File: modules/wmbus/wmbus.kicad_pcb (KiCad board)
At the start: 2 copper layers, 25.4 x 28.6 mm, 15 parts, among them J1 Conn_01x08, J2 Conn_01x08, U2 RC-S2LP-868

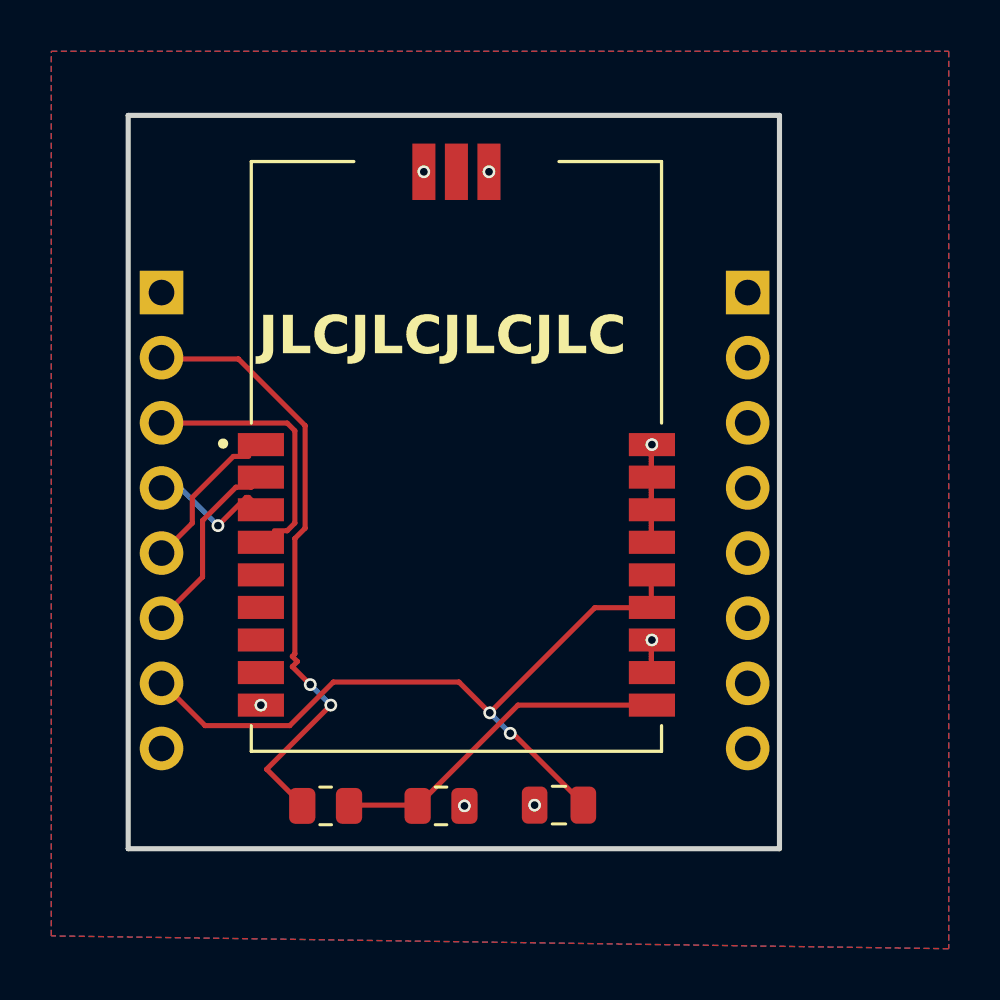
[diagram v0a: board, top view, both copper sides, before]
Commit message: cross check wmbus module is ready for fabrication
Signed-off-by: Rodney Osodo <socials@rodneyosodo.com>
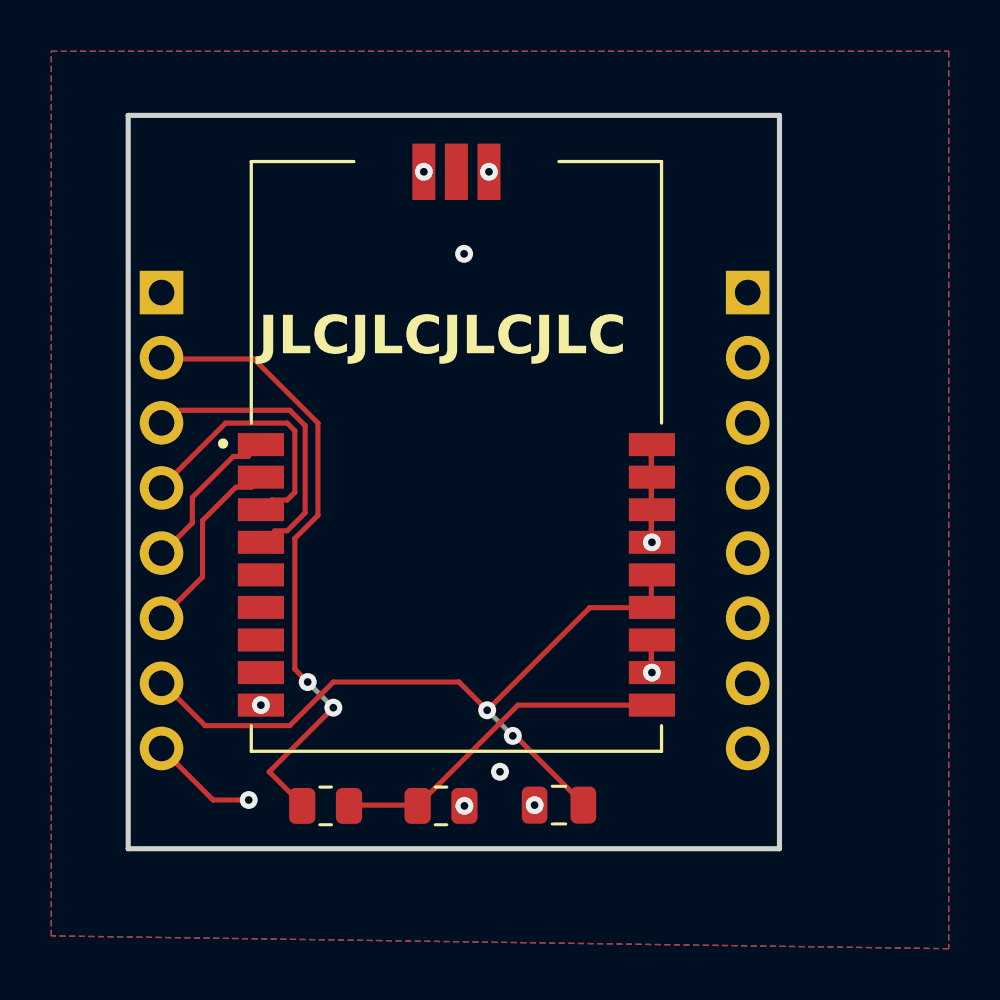
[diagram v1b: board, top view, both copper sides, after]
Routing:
- net SCK: track 5.22 -> 10.4 mm, vias 1 -> 0
- net GND: track 5.41 -> 9.64 mm, vias 7 -> 10
- net CS: track 9.90 -> 11.0 mm
- net SDN: track 24.1 -> 24.6 mm
